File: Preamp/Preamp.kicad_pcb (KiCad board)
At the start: 2 copper layers, 83 x 54 mm, 55 parts, among them J1 +20, J10 R Out+, J11 R Out-, J2 GND, J3 -20, J4 L In+, J5 L In-, J6 R In+, J7 R In-, J8 L Out+, J9 L Out-, U1 L7815, U2 L7915, U3 OPA2134, U4 OPA2134

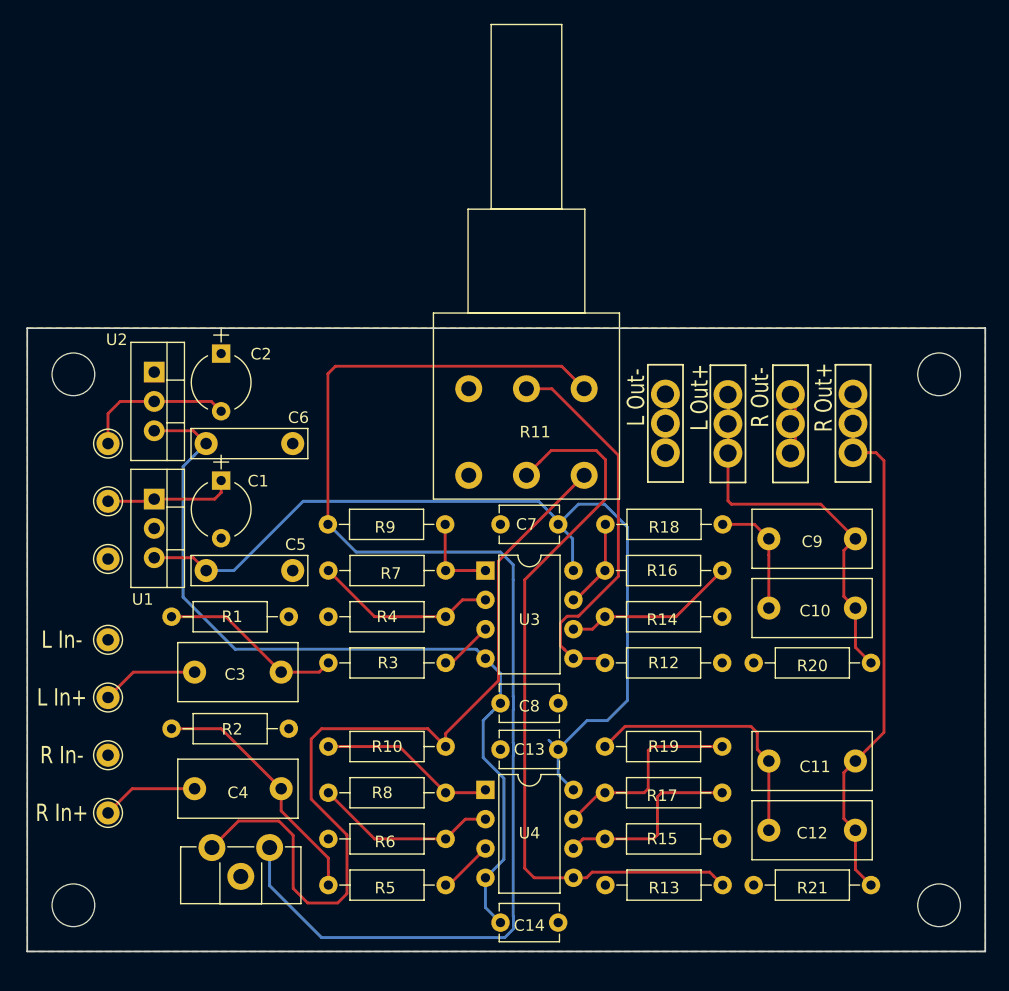
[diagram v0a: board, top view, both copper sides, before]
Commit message: fixed libraries, now works everything, including 3d models
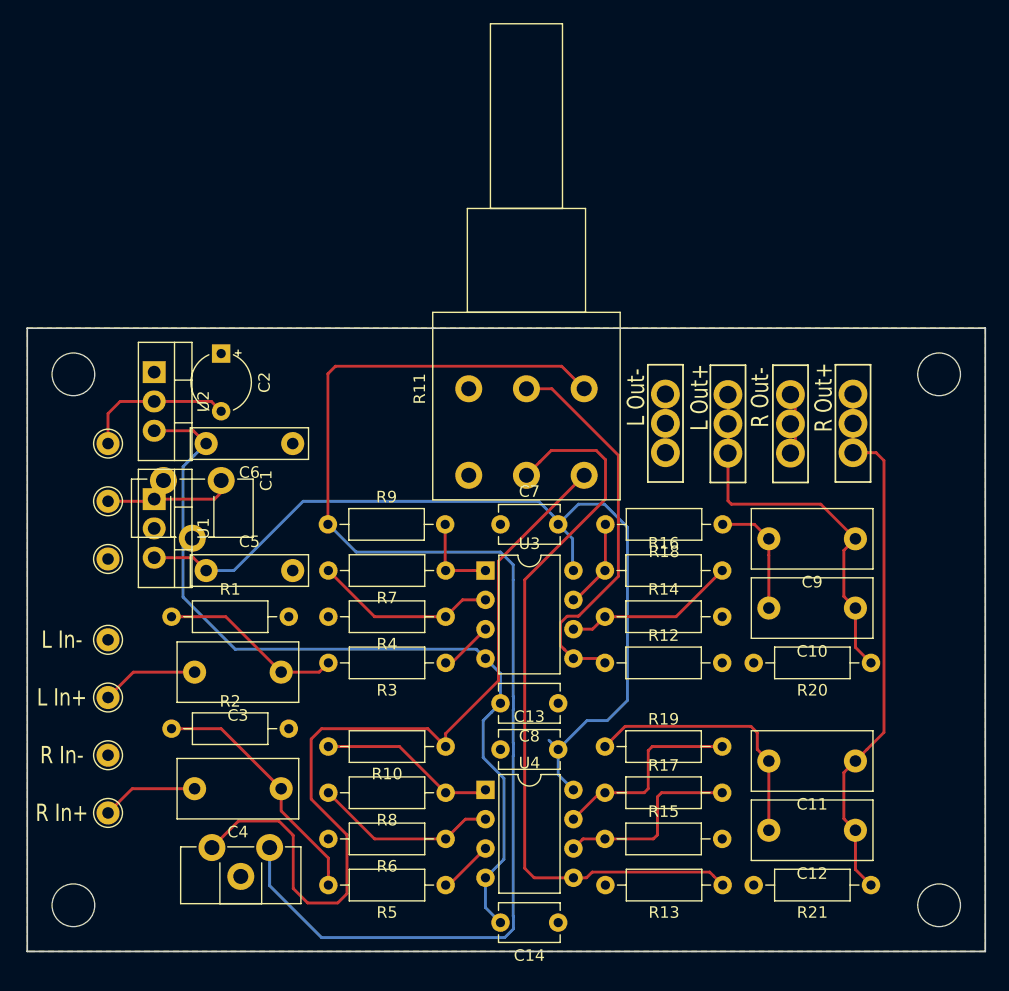
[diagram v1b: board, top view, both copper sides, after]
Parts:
- C1: footprint Capacitors_THT:CP_Radial_Tantal_D5.0mm_P5.00mm -> Potentiometer_THT:Potentiometer_Piher_PT-10-H05_Horizontal
- C10, C11, C12, C3, C4, C9: footprint Capacitors_THT:C_Rect_L10.3mm_W5.0mm_P7.50mm_MKS4 -> Capacitor_THT:C_Rect_L10.3mm_W5.0mm_P7.50mm_MKS4
- C13, C14, C7, C8: footprint Capacitors_THT:C_Disc_D5.1mm_W3.2mm_P5.00mm -> Capacitor_THT:C_Disc_D5.1mm_W3.2mm_P5.00mm
- C2: footprint Capacitors_THT:CP_Radial_Tantal_D5.0mm_P5.00mm -> Capacitor_THT:CP_Radial_Tantal_D5.0mm_P5.00mm
- C5, C6: footprint Capacitors_THT:C_Rect_L10.0mm_W2.5mm_P7.50mm_MKS4 -> Capacitor_THT:C_Rect_L10.0mm_W2.5mm_P7.50mm_MKS4
- R1, R10, R12, R13, R14, R15, R16, R17, R18, R19, R2, R20, R21, R3, R4, R5, R6, R7, R8, R9: footprint Resistors_THT:R_Axial_DIN0207_L6.3mm_D2.5mm_P10.16mm_Horizontal -> Resistor_THT:R_Axial_DIN0207_L6.3mm_D2.5mm_P10.16mm_Horizontal
- R11: footprint Potentiometers:Potentiometer_Piher_PC-16_Double_Vertical -> Potentiometer_THT:Potentiometer_Piher_PC-16_Dual_Horizontal
- U1, U2: footprint TO_SOT_Packages_THT:TO-220-3_Vertical -> Package_TO_SOT_THT:TO-220-3_Vertical
- U3, U4: footprint Housings_DIP:DIP-8_W7.62mm -> Package_DIP:DIP-8_W7.62mm
